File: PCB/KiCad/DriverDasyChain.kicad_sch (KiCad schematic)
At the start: 34 parts, among them J1 Conn_01x02, J10 Conn_01x06, J11 Conn_01x07_Socket, J12 Conn_01x03, J13 Conn_01x03, J16 Conn_01x02, J2 Conn_01x02, J4 Conn_01x04, J5 Conn_01x03, J7 Conn_01x07_Pin, J8 Conn_01x07_Pin, J9 Conn_01x07_Socket, Q2 Q_NMOS_GDS, SW2 SW_DPST_x2, U1 AP2112K-3.3, U2 XIAO-ESP32-S3-DIP, U3 74AHCT1G125, U4 SN65HVD230

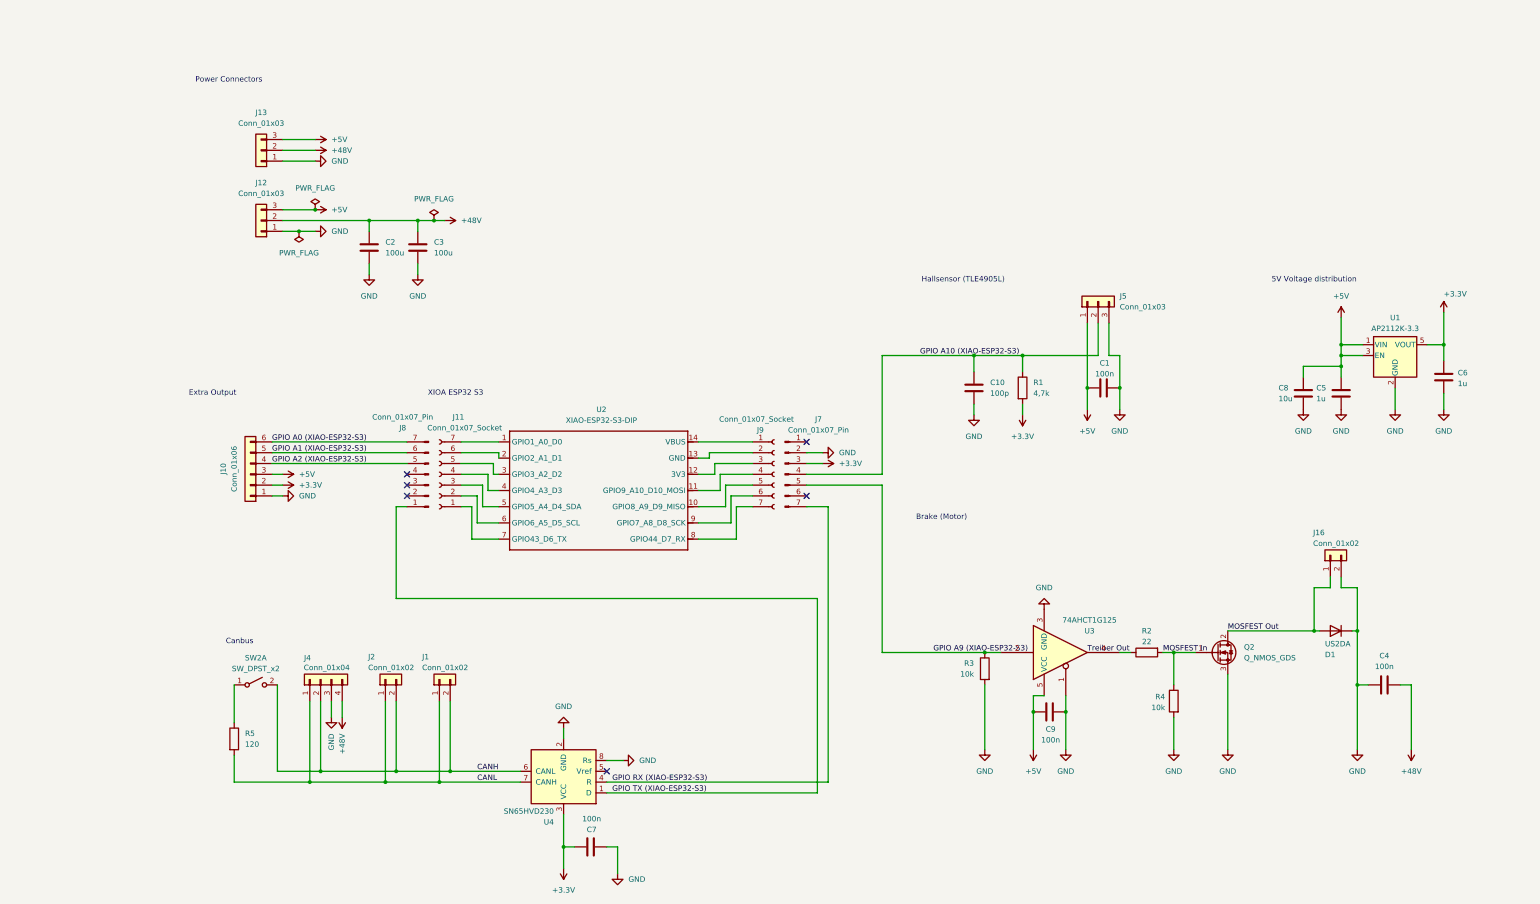
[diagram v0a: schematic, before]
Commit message: Keine Änderungen vorgenommen.
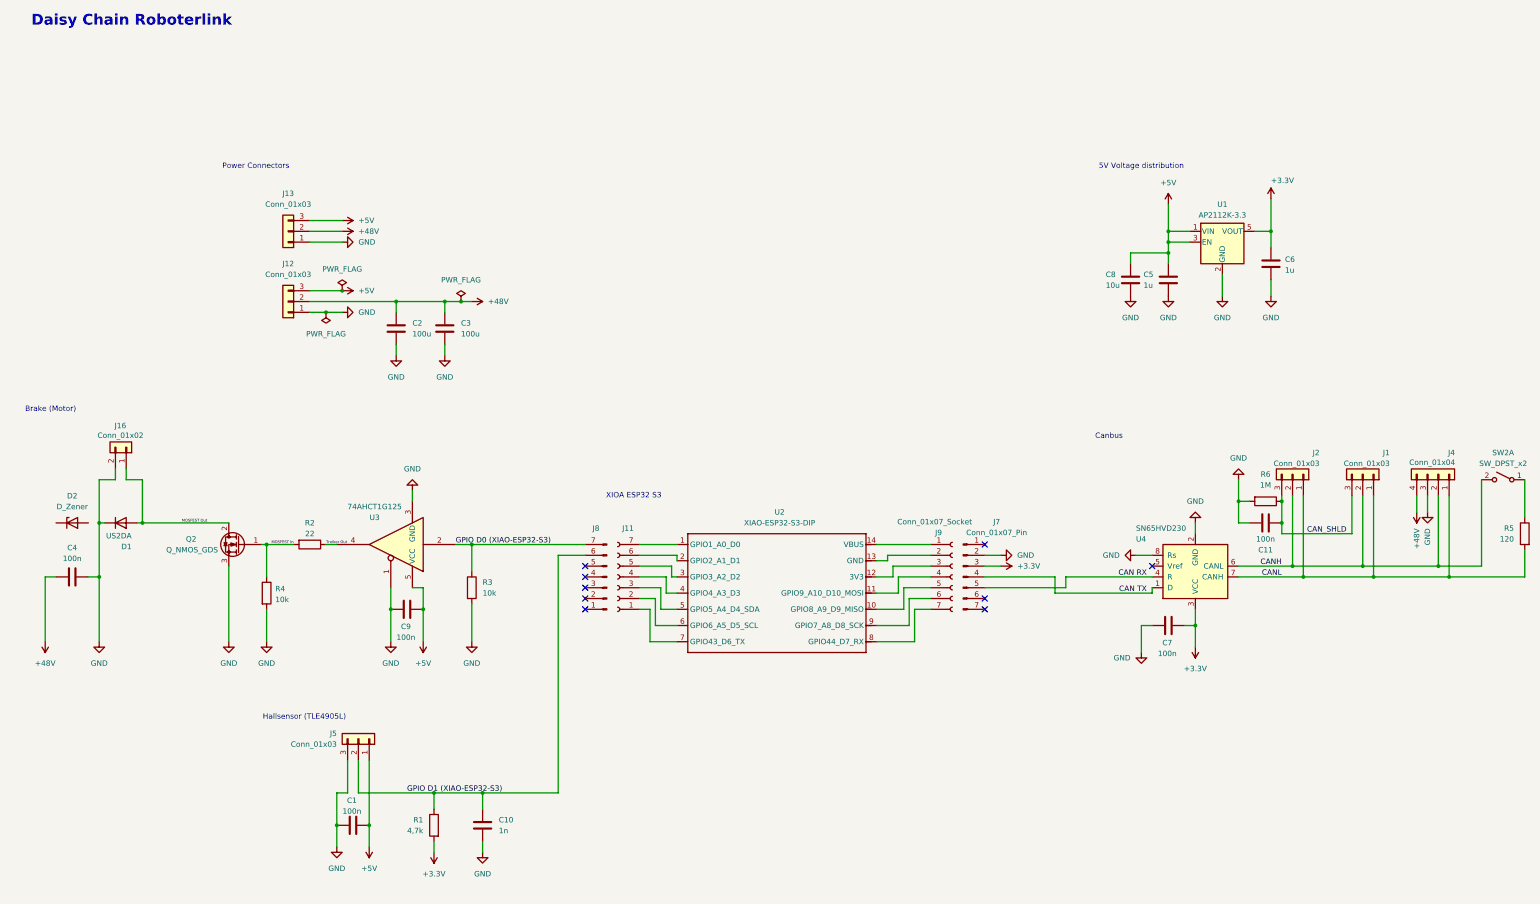
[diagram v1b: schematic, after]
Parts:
- removed J1, J2: Conn_01x02, Connector_Molex:Molex_Micro-Fit_3.0_43650-0300_1x03_P3.00mm_Horizontal, symbol Connector_Generic:Conn_01x02
- removed J10: Conn_01x06, Connector_JST:JST_XH_B6B-XH-A_1x06_P2.50mm_Vertical, symbol Connector_Generic:Conn_01x06
- added C11: 100n, symbol Device:C
- added D2: D_Zener, symbol Device:D_Zener
- added J1, J2: Conn_01x03, Connector_Molex:Molex_Micro-Fit_3.0_43650-0300_1x03_P3.00mm_Horizontal, symbol Connector_Generic:Conn_01x03
- added R6: 1M, symbol Device:R
- C10: value 100p -> 1n
- R5: footprint (none) -> Resistor_SMD:R_0603_1608Metric_Pad0.98x0.95mm_HandSolder
- SW2: footprint (none) -> Button_Switch_SMD:SW_DIP_SPSTx01_Slide_6.7x4.1mm_W6.73mm_P2.54mm_LowProfile_JPin
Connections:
- net GPIO A0 (XIAO-ESP32-S3) is gone; now on net GPIO D0 (XIAO-ESP32-S3): J8.7 (Pin_7)
- net GPIO A1 (XIAO-ESP32-S3) is gone; now on an unnamed net: J8.6 (Pin_6)
- net CANH: now also J1.2 (Pin_2), J2.2 (Pin_2)
- net CANL: now also J1.1 (Pin_1), J2.1 (Pin_1)
- net GND: now also C11.1, R6.2
- net Treiber Out: now also R2.1, U3.4
- net at C10.1, J5.2 (Pin_2), Q2.1 (G)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: no longer J7.4 (Pin_4)
- net GPIO D0 (XIAO-ESP32-S3): now reaches R3.1, U3.2
- net GPIO D0 (XIAO-ESP32-S3): no longer J7.5 (Pin_5)
- net GPIO A2 (XIAO-ESP32-S3): no longer names the net of J8.5 (Pin_5)
- net GPIO RX (XIAO-ESP32-S3): no longer names the net of J7.7 (Pin_7)
- net GPIO RX (XIAO-ESP32-S3): no longer U4.4 (R)
- net GPIO TX (XIAO-ESP32-S3): no longer names the net of J8.1 (Pin_1)
- net GPIO TX (XIAO-ESP32-S3): no longer U4.1 (D)
- new net CAN RX: J7.5 (Pin_5), U4.4 (R)
- new net CAN TX: J7.4 (Pin_4), U4.1 (D)
- new net CAN_SHLD: C11.2, J1.3 (Pin_3), J2.3 (Pin_3), R6.1
- no-connect marks 6 -> 9
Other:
- note added: "Daisy Chain Roboterlink"
- note removed: "Extra Output"
- moved on the sheet: C1, C10, C2, C3, C4, C5, C6, C7, C8, C9, D1, J11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
